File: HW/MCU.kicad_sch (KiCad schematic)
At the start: 7 parts, among them U6 STM32C031KxTx, U7 STM32C031KxUx

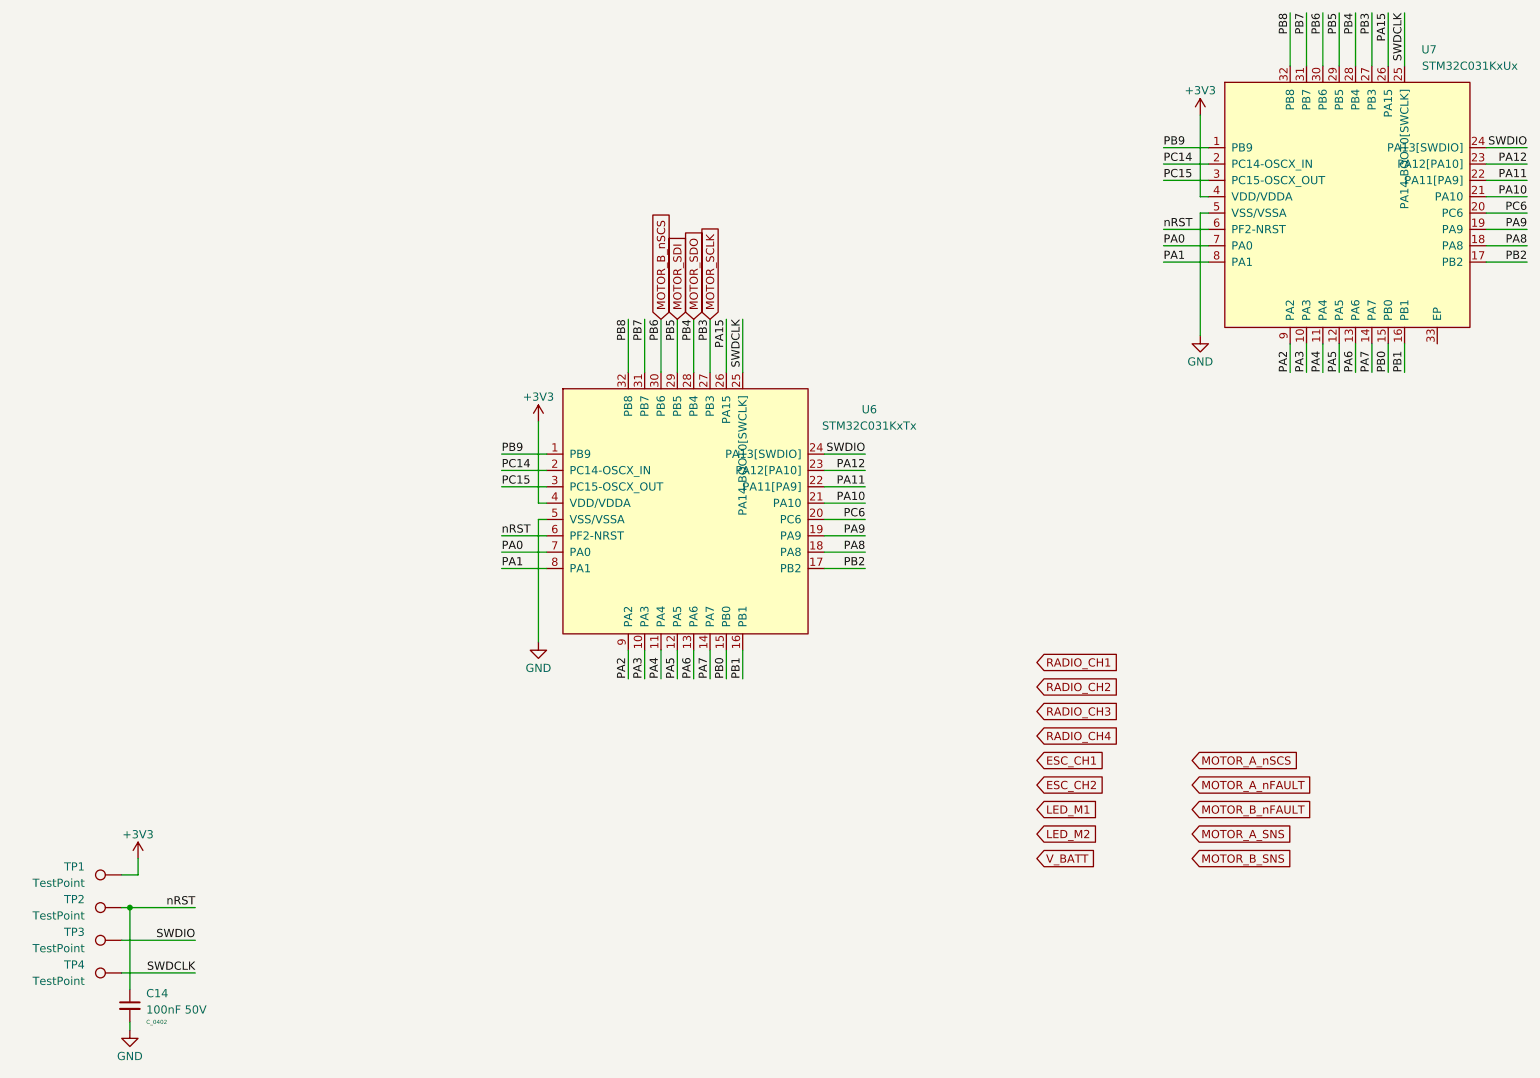
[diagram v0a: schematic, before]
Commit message: WIP - Final Detail Design Before Design Review
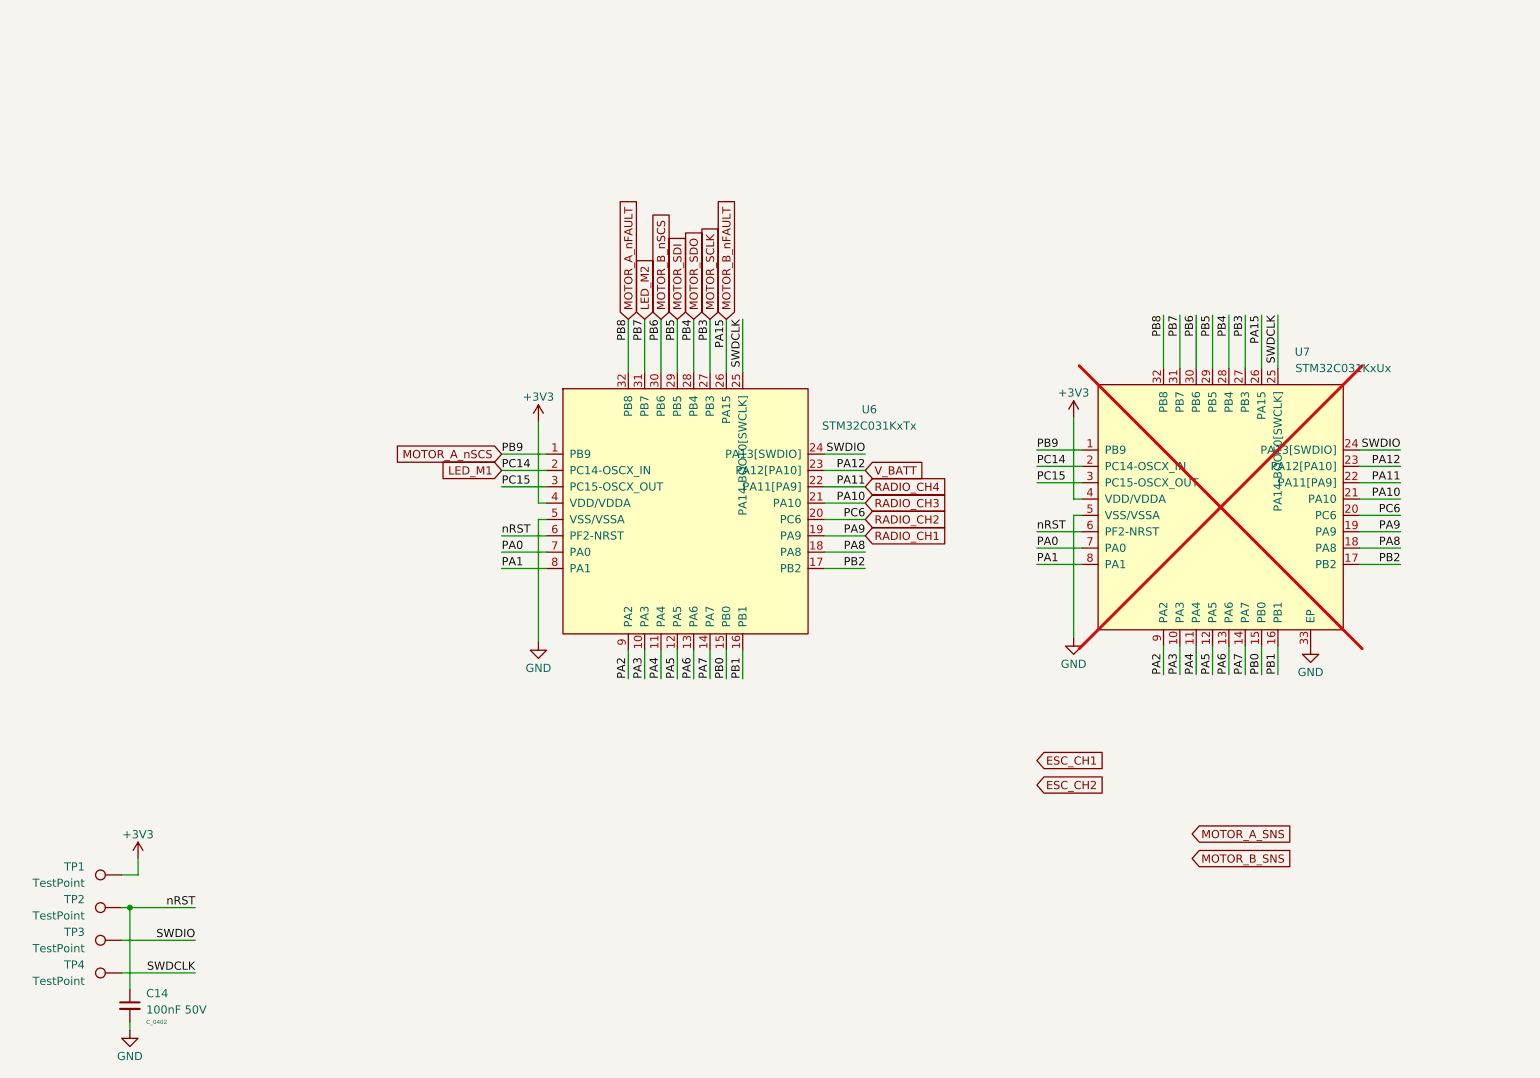
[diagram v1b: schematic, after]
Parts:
- U7: now not fitted
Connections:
- net PA10 is gone; now on net RADIO_CH3: U6.21 (PA10), U7.21 (PA10)
- net PA11 is gone; now on net RADIO_CH4: U6.22 (PA11[PA9]), U7.22 (PA11[PA9])
- net PA12 is gone; now on net V_BATT: U6.23 (PA12[PA10]), U7.23 (PA12[PA10])
- net PA15 is gone; now on net MOTOR_B_nFAULT: U6.26 (PA15), U7.26 (PA15)
- net PA9 is gone; now on net RADIO_CH1: U6.19 (PA9), U7.19 (PA9)
- net PB7 is gone; now on net LED_M2: U6.31 (PB7), U7.31 (PB7)
- net PB8 is gone; now on net MOTOR_A_nFAULT: U6.32 (PB8), U7.32 (PB8)
- net PB9 is gone; now on net MOTOR_A_nSCS: U6.1 (PB9), U7.1 (PB9)
- net PC14 is gone; now on net LED_M1: U6.2 (PC14-OSCX_IN), U7.2 (PC14-OSCX_IN)
- net PC6 is gone; now on net RADIO_CH2: U6.20 (PC6), U7.20 (PC6)
- net GND: now also U7.33 (EP)
